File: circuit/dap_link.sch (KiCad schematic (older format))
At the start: 18 parts, among them J1 USB_A, U1 STM32F103CBTx, U2 AMS1117-3.3, Y1 8MHz

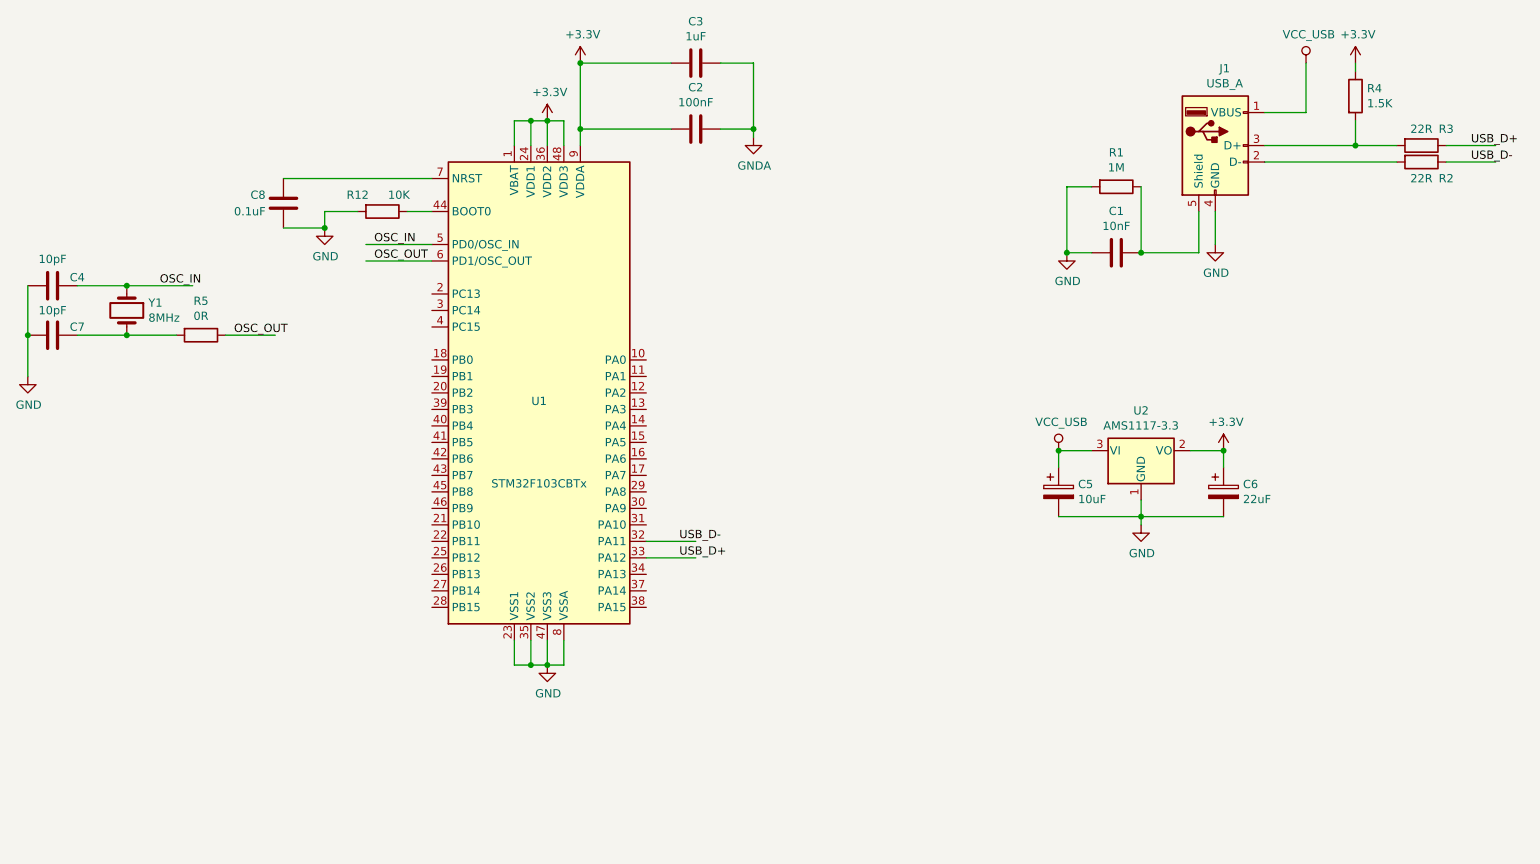
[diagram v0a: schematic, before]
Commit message: footprint done
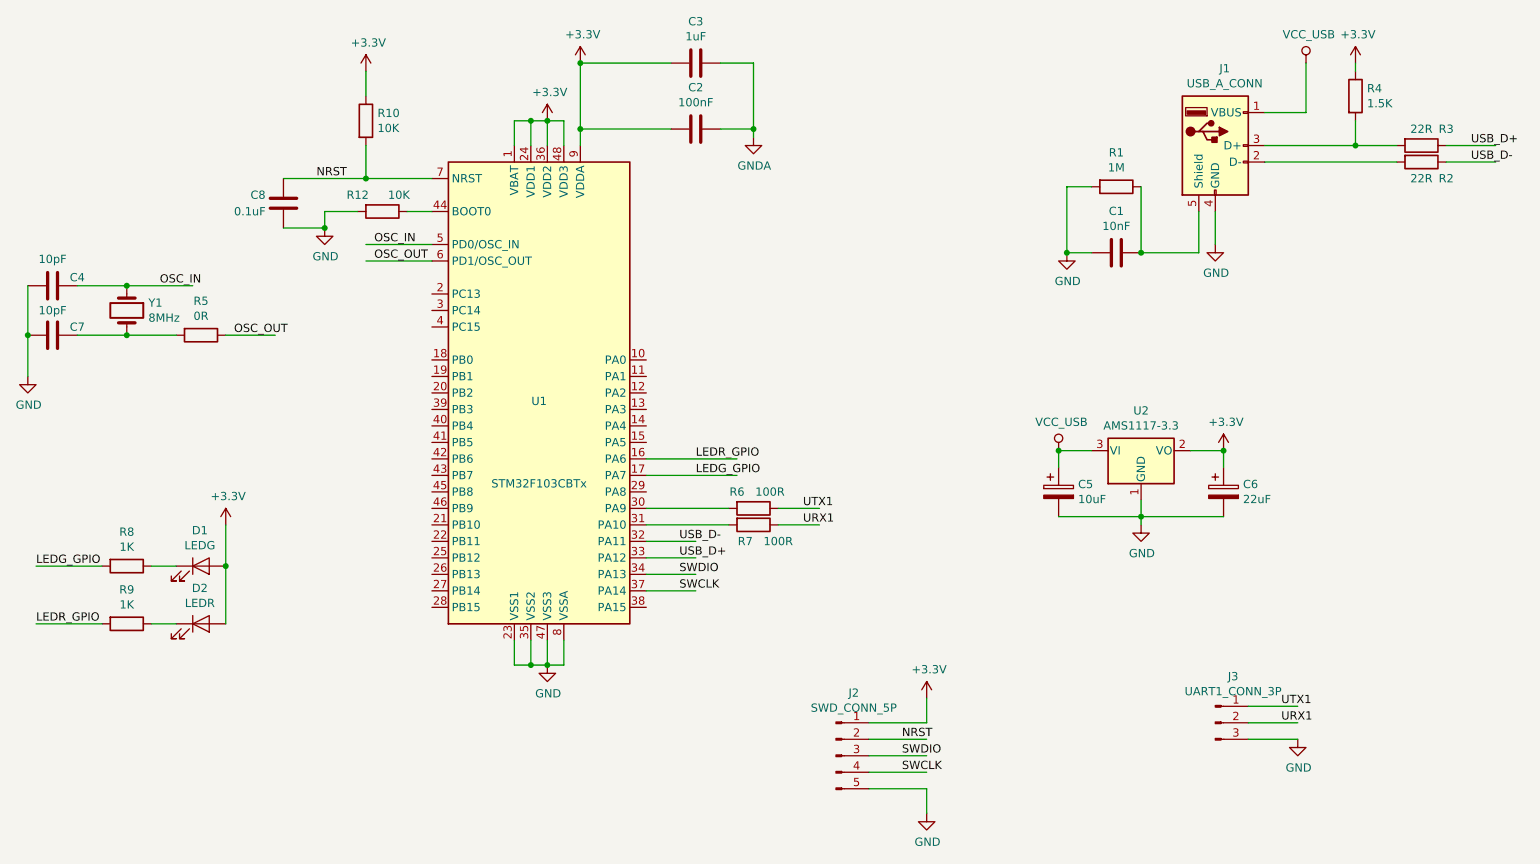
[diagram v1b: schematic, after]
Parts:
- added D1: LEDG, LED_SMD:LED_0603_1608Metric_Pad1.05x0.95mm_HandSolder, symbol Device:LED
- added D2: LEDR, LED_SMD:LED_0603_1608Metric_Pad1.05x0.95mm_HandSolder, symbol Device:LED
- added J2: SWD_CONN_5P, Connector_PinHeader_2.54mm:PinHeader_1x05_P2.54mm_Vertical, symbol Connector:Conn_01x05_Male
- added J3: UART1_CONN_3P, Connector_PinHeader_2.54mm:PinHeader_1x03_P2.54mm_Vertical, symbol Connector:Conn_01x03_Male
- added R10: 10K, Resistor_SMD:R_0603_1608Metric_Pad1.05x0.95mm_HandSolder, symbol Device:R
- added R6, R7: 100R, Resistor_SMD:R_0603_1608Metric_Pad1.05x0.95mm_HandSolder, symbol Device:R
- added R8, R9: 1K, Resistor_SMD:R_0603_1608Metric_Pad1.05x0.95mm_HandSolder, symbol Device:R
- C1, C2, C3, C4, C7, C8: footprint (none) -> Capacitor_SMD:C_0603_1608Metric_Pad1.05x0.95mm_HandSolder
- C5, C6: footprint (none) -> Capacitor_Tantalum_SMD:CP_EIA-3528-12_Kemet-T_Pad1.50x2.35mm_HandSolder
- J1: value USB_A -> USB_A_CONN; footprint (none) -> Connector_USB:USB_A_CNCTech_1001-011-01101_Horizontal
- R1, R12, R2, R3, R4, R5: footprint (none) -> Resistor_SMD:R_0603_1608Metric_Pad1.05x0.95mm_HandSolder
- Y1: footprint (none) -> Crystal:Crystal_SMD_SeikoEpson_MA505-2Pin_12.7x5.1mm
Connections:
- net labels added: LEDG_GPIO, LEDR_GPIO, NRST, SWCLK, SWDIO, URX1, UTX1
- wire segments 62 -> 89
